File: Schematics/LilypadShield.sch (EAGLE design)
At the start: 38 parts, among them T1 , T2 

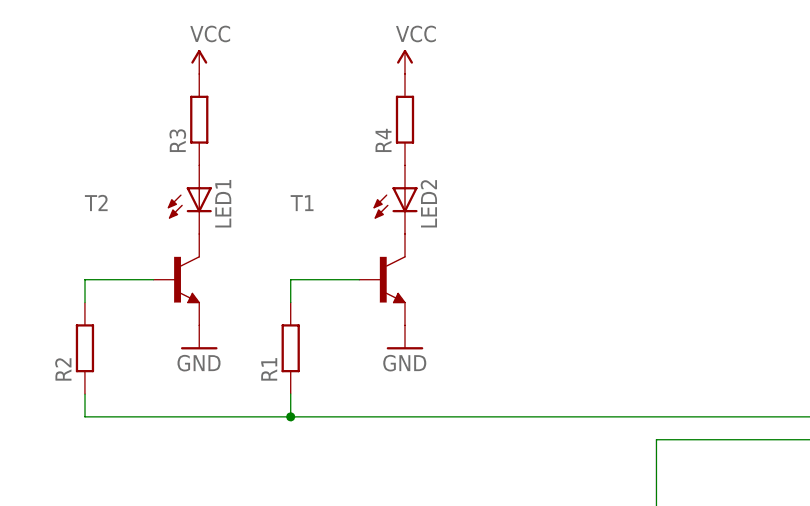
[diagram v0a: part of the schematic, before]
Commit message: NanoShield
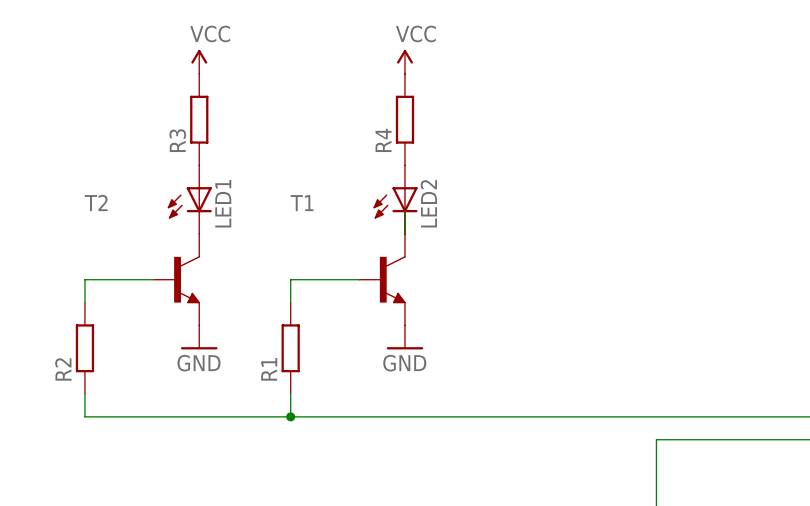
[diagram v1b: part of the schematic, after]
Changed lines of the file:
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@@
+</segment>
+</net>
+<net name="N$8" class="0">
+<segment>
+<wire x1="101.6" y1="160.02" x2="101.6" y2="162.56" width="0.1524" layer="91"/>
 </segment>
 </net>
